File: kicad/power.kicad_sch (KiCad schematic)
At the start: 54 parts, among them J1 L, J2 N, J3 PE, J4 PE, J5 VOUT+, J6 VOUT-, Q5 BD677, U2 AP64060QWU, U3 AP64060QWU

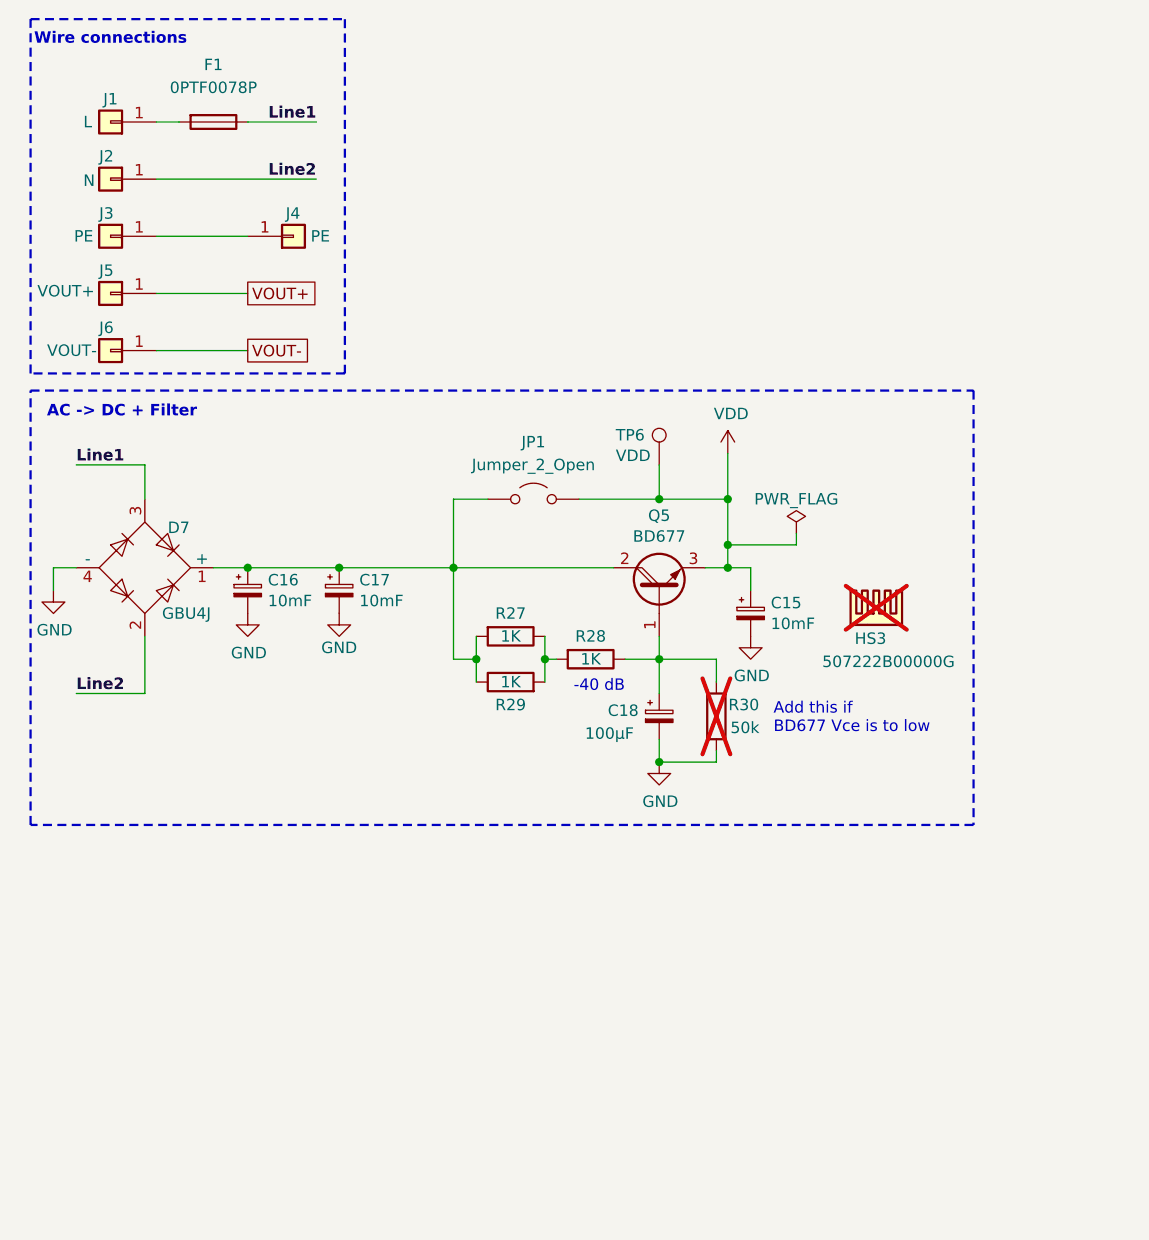
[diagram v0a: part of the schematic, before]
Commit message: Commit
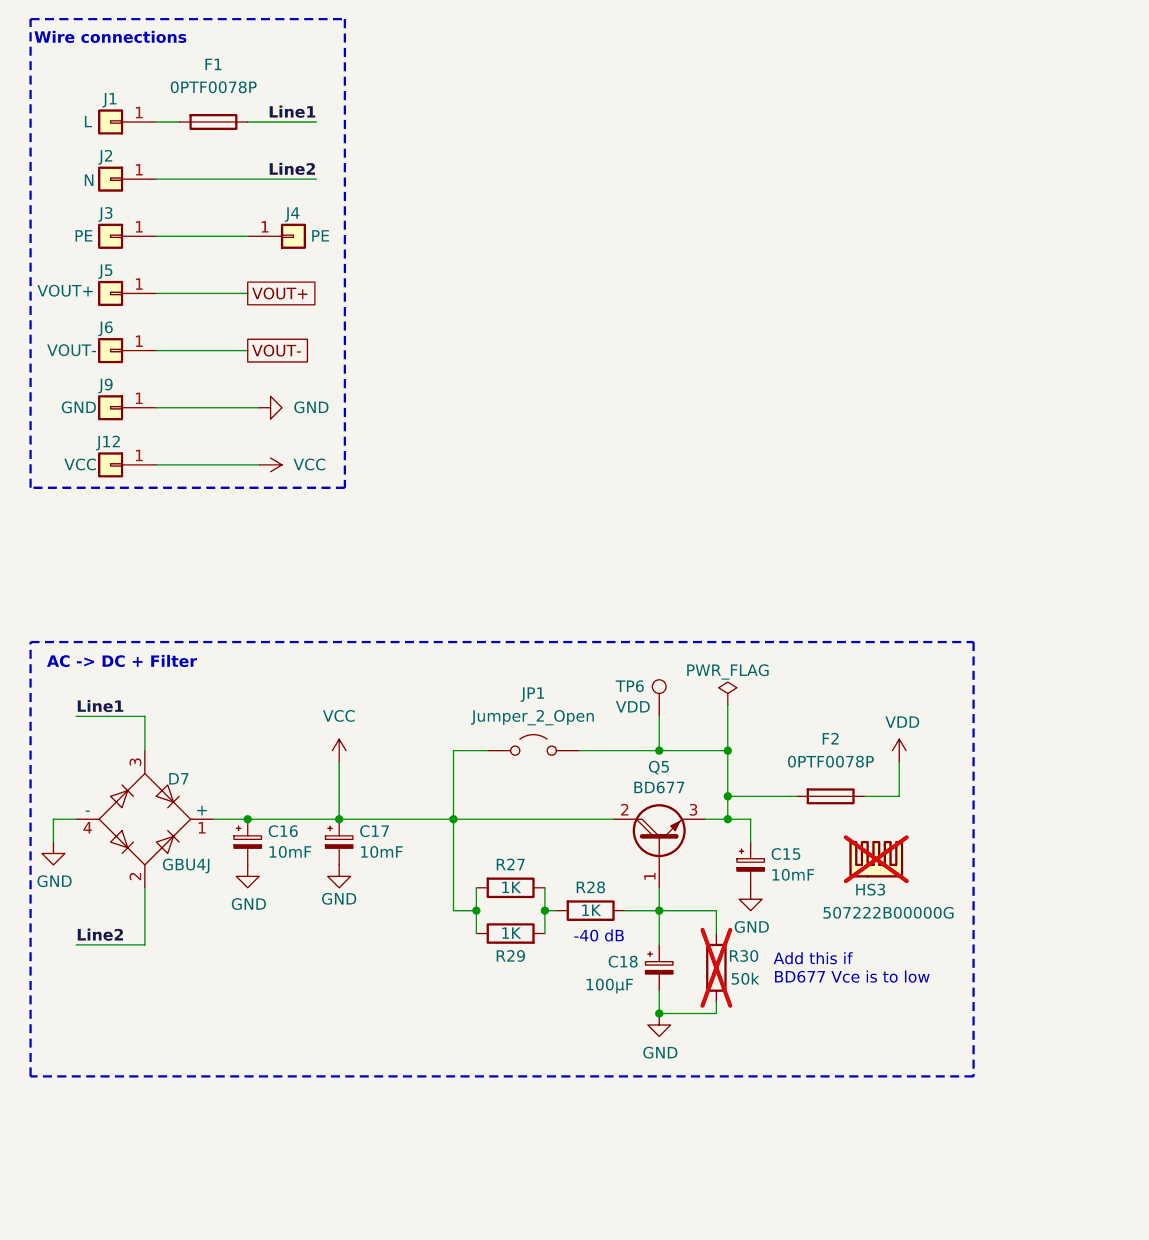
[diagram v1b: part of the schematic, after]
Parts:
- added F2: 0PTF0078P, footprints:FuseHolder, symbol Device:Fuse
- added J12: VCC, TestPoint:TestPoint_Pad_4.0x4.0mm, symbol Connector_Generic:Conn_01x01
- added J9: GND, TestPoint:TestPoint_Pad_4.0x4.0mm, symbol Connector_Generic:Conn_01x01
- C13, C21: MPN CL21B105KBFNNNF -> CL21B105KBFNNNF
- C22, C56: MPN CL31A106KBHNNNE -> CL31A106KBHNNNE
- JP1, TP6: now left out of the parts list
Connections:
- net GND: now also J9.1 (Pin_1)
- net VDD: now also F2.1; no longer C15.1, JP1.2 (B), Q5.3 (E), TP6.1
- net VCC: now reaches C16.1, C17.1, D7.1 (+), JP1.1 (A), Q5.2 (C), R27.2, R29.1
- net VCC: now also J12.1 (Pin_1)
- new net: C15.1, F2.2, JP1.2 (B), Q5.3 (E), TP6.1
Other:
- moved on the sheet: C15, C16, C17, C18, D7, HS3, JP1, Q5, R27, R28, R29, R30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
